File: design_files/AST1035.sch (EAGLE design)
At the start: 4 parts, among them J1 SM05B, J5 AST7525, Q1 2N7002P

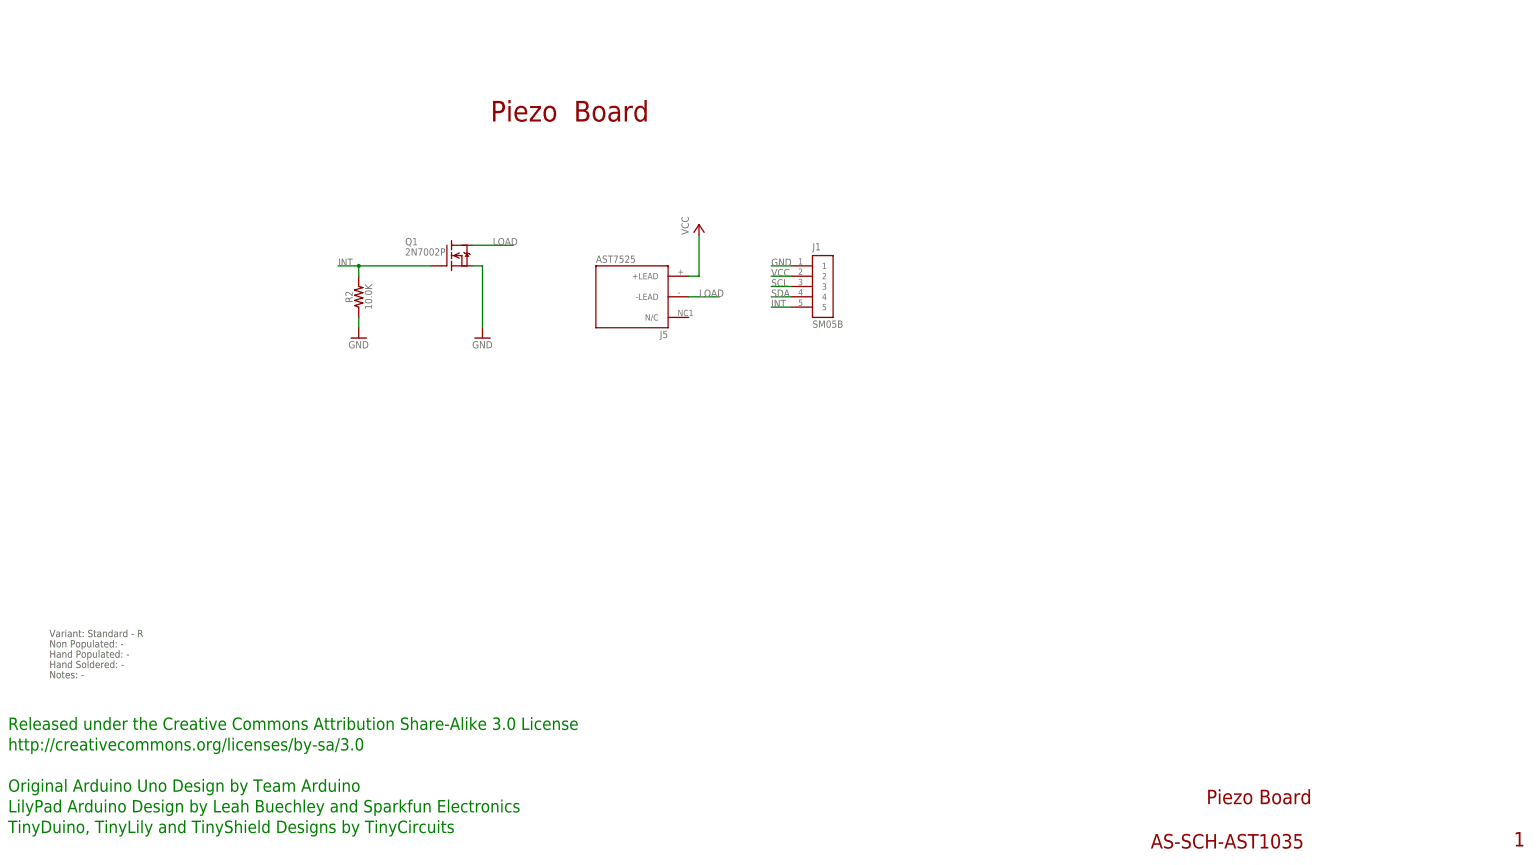
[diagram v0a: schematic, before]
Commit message: update naming
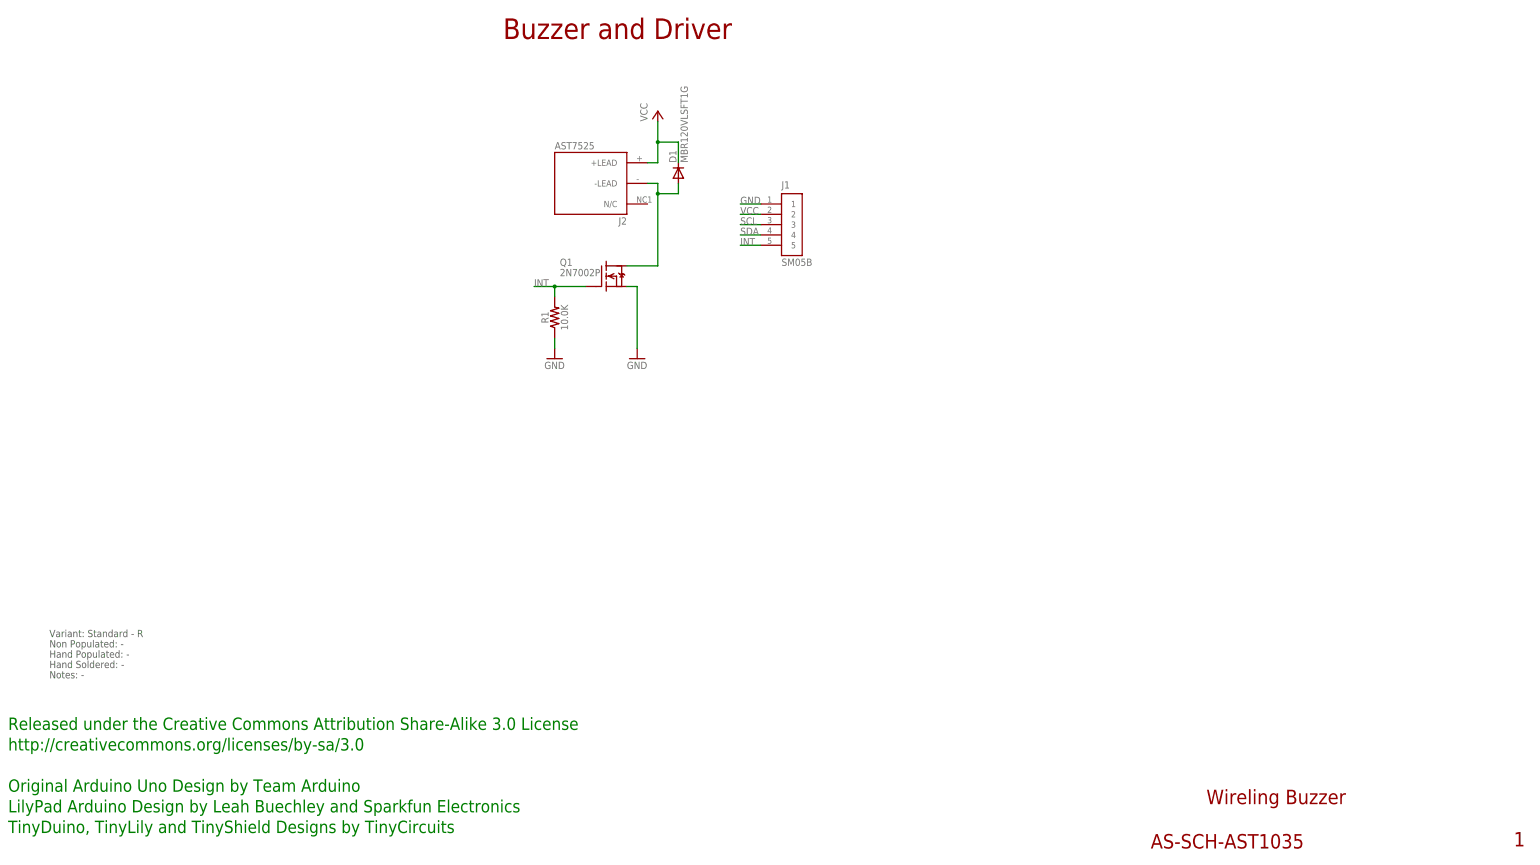
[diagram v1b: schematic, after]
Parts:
- removed J5: AST7525, tinycircuits:AS-ITM-00390
- removed R2: 10.0K, tinycircuits:AS-ITM-00032
- added D1: MBR120VLSFT1G, tinycircuits:AS-ITM-00111
- added J2: AST7525, tinycircuits:AS-ITM-00390
- added R1: 10.0K, tinycircuits:AS-ITM-00032
- J1: device tinycircuits:AS-ITM-00340 -> tinycircuits:AS-ITM-00340EDGE
- Q1: device tinycircuits:AS-ITM-00007 -> tinycircuits:AS-ITM-00007C
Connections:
- net GND: now also R1.1; no longer R2.1
- net INT: now also R1.2; no longer R2.2
- net LOAD: now also D1.A, J2.-LEAD; no longer J5.-LEAD
- net VCC: now also D1.C, J2.+LEAD; no longer J5.+LEAD
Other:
- note added: "Buzzer and Driver"
- note added: "Wireling Buzzer"
- note removed: "Piezo Board"
- moved on the sheet: J1, Q1
